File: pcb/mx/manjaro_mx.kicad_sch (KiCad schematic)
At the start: 97 parts, among them SW1 SW_Push, SW10 SW_Push, SW11 SW_Push, SW12 SW_Push, SW13 SW_Push, SW14 SW_Push, SW15 SW_Push, SW16 SW_Push, SW17 SW_Push, SW18 SW_Push, SW19 SW_Push, SW2 SW_Push, SW20 SW_Push, SW21 SW_Push, SW22 SW_Push, SW3 SW_Push, SW4 SW_Push, SW5 SW_Push, SW6 SW_Push, SW7 SW_Push, SW8 SW_Push, SW9 SW_Push, U1 nice_nano

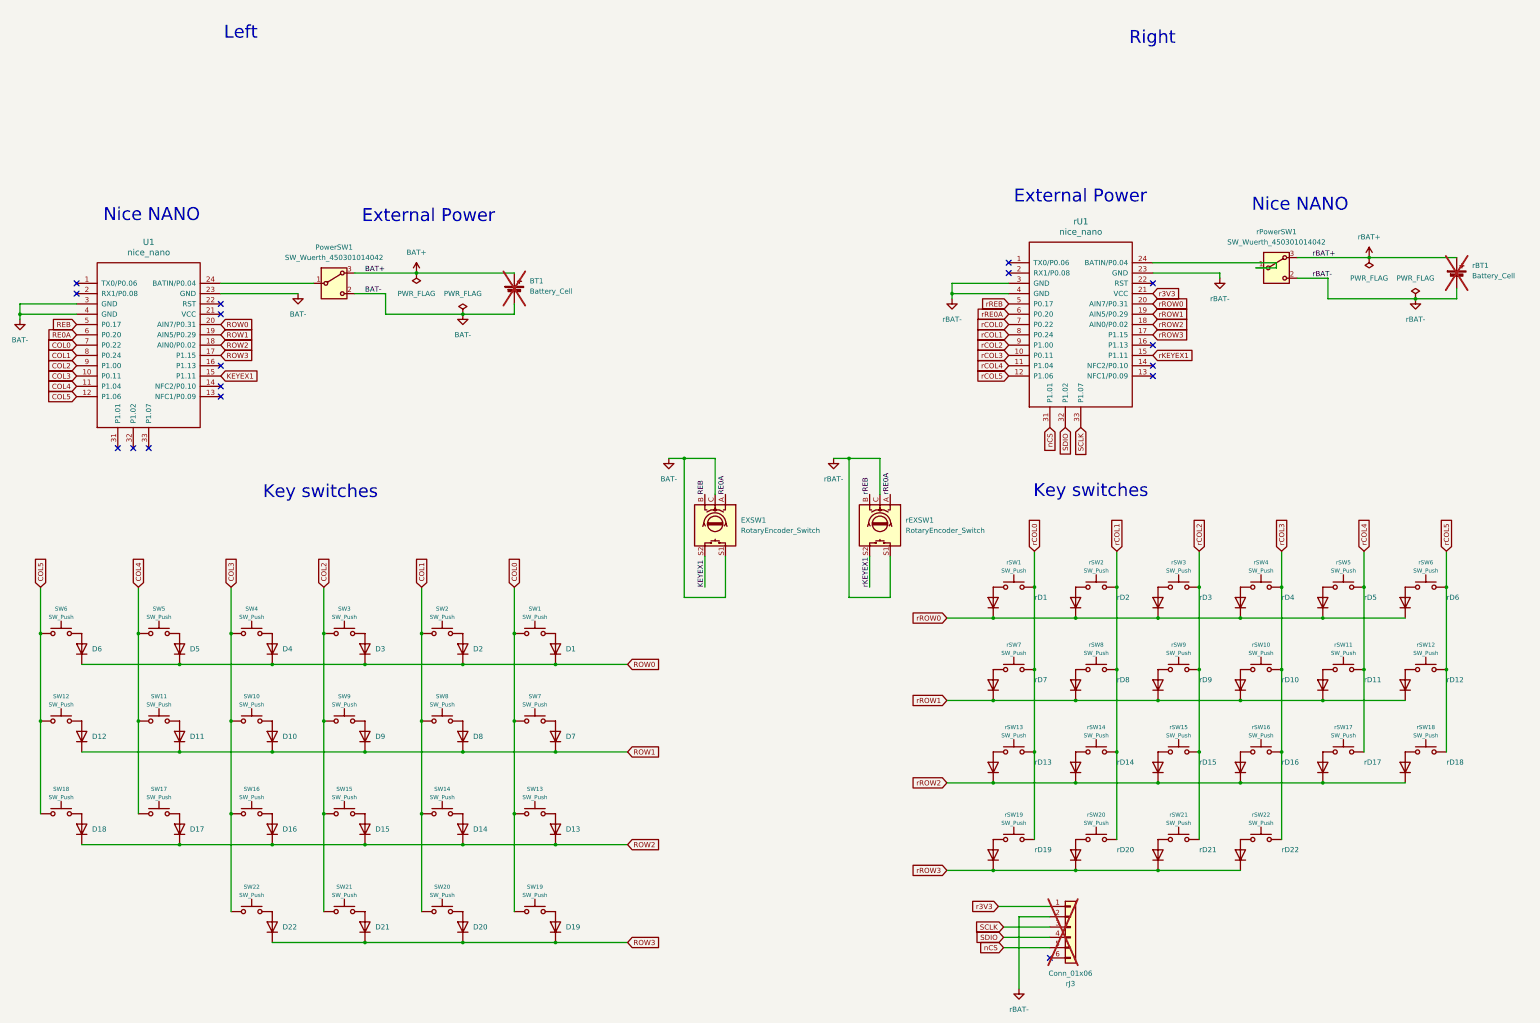
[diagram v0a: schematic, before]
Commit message: Fixed v1 layout
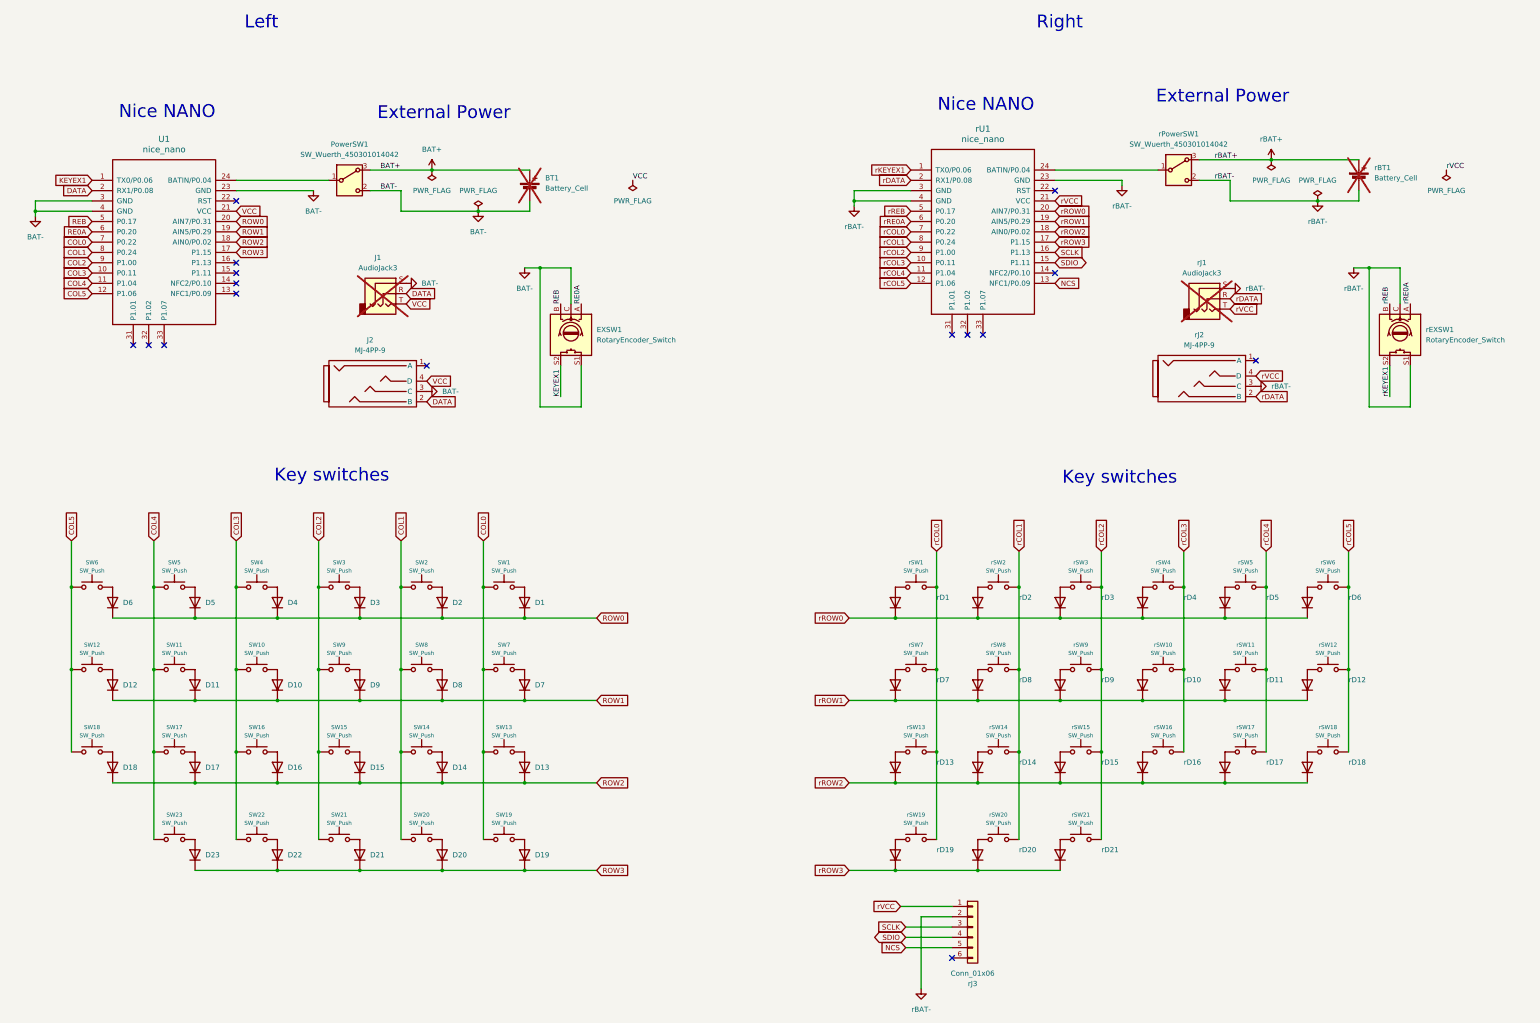
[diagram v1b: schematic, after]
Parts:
- removed rD22: 1N4148WT, Keebio-Parts:D_SOD-323, symbol Diode:1N4148WT
- removed rSW22: SW_Push, kbd_SW:Choc_Hotswap_1u, symbol Switch:SW_Push
- added D23: 1N4148WT, Keebio-Parts:D_SOD-323, symbol Diode:1N4148WT
- added J1, rJ1: AudioJack3, kbd:PJ-398A-5A_PJ-399B-6A, symbol Connector_Audio:AudioJack3
- added J2, rJ2: MJ-4PP-9, MJ-4PP-9:MJ-4PP-9, symbol MJ-4PP-9:MJ-4PP-9
- added SW23: SW_Push, kbd:keyswitch_cherrymx_hotswap_1u, symbol Switch:SW_Push
- SW1, SW10, SW11, SW12, SW13, SW14, SW15, SW16, SW17, SW18, SW19, SW2, SW20, SW21, SW22, SW3, SW4, SW5, SW6, SW7, SW8, SW9, rSW1, rSW10, rSW11, rSW12, rSW13, rSW14, rSW15, rSW16, rSW17, rSW18, rSW19, rSW2, rSW20, rSW21, rSW3, rSW4, rSW5, rSW6, rSW7, rSW8, rSW9: footprint kbd_SW:Choc_Hotswap_1u -> kbd:keyswitch_cherrymx_hotswap_1u
- rJ3: now fitted
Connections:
- net BAT-: now also J1.S, J2.3 (C)
- net COL4: now also SW23.1
- net KEYEX1: now also U1.1 (TX0/P0.06); no longer U1.15 (P1.11)
- net ROW3: now also D23.1 (K)
- net SCLK: now also rU1.16 (P1.13); no longer rU1.33 (P1.07)
- net SDIO: now also rU1.15 (P1.11); no longer rU1.32 (P1.02)
- net rBAT-: now also rJ1.S, rJ2.3 (C)
- net rKEYEX1: now also rU1.1 (TX0/P0.06); no longer rU1.15 (P1.11)
- net NCS: now reaches rU1.13 (NFC1/P0.09)
- net NCS: now also rJ3.5 (Pin_5)
- net rDATA: now reaches rU1.2 (RX1/P0.08)
- net rDATA: now also rJ1.R, rJ2.2 (B)
- net DATA: now reaches U1.2 (RX1/P0.08)
- net DATA: now also J1.R, J2.2 (B)
- net VCC: now reaches U1.21 (VCC)
- net VCC: now also J1.T, J2.4 (D)
- net nCS: no longer names the net of rU1.31 (P1.01)
- net nCS: no longer rJ3.5 (Pin_5)
- net r3V3 renamed rVCC
- net rVCC: now also rJ1.T, rJ2.4 (D)
- new net: D23.2 (A), SW23.2
- no-connect marks 17 -> 16
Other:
- moved on the sheet: BT1, D1, D10, D11, D12, D13, D14, D15, D16, D17, D18, D19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
